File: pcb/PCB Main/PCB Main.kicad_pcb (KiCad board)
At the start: 4 copper layers, 64.1 x 56.5 mm, 81 parts, among them CN1 Conn_01x07, CN2 Conn_01x02, CN3 Conn_01x02, CN4 Conn_01x04, CN5 Conn_01x04, CN6 Conn_01x03, CN7 Conn_01x03, CN8 Conn_01x03, CN9 Conn_01x02, J1 Conn_01x03, Q1 AO3401A, SW1 SW_Reset, U1 STM32WB55RGVx, U2 AEM10941, U3 INA3221, U4 MB85RS256B, X1 32MHz, X2 32.768kHz

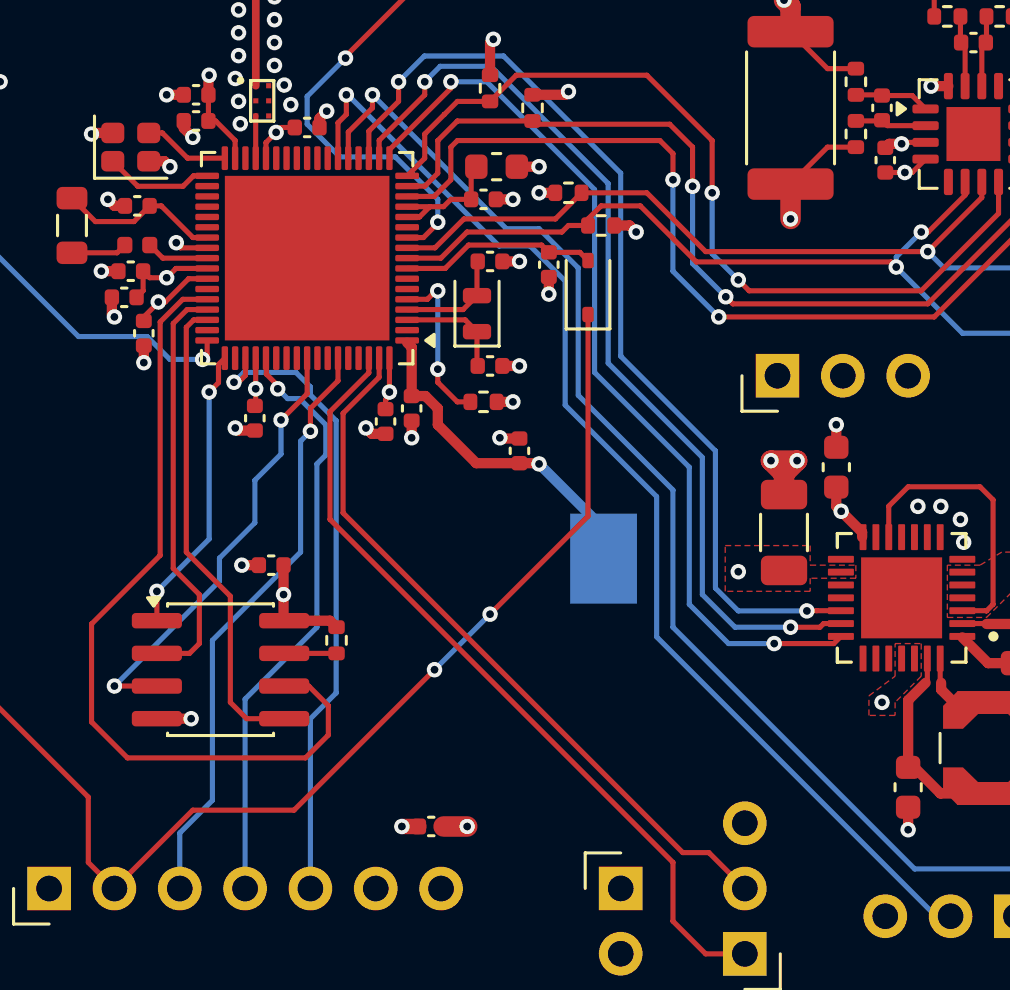
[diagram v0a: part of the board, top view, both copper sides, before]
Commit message: retoques
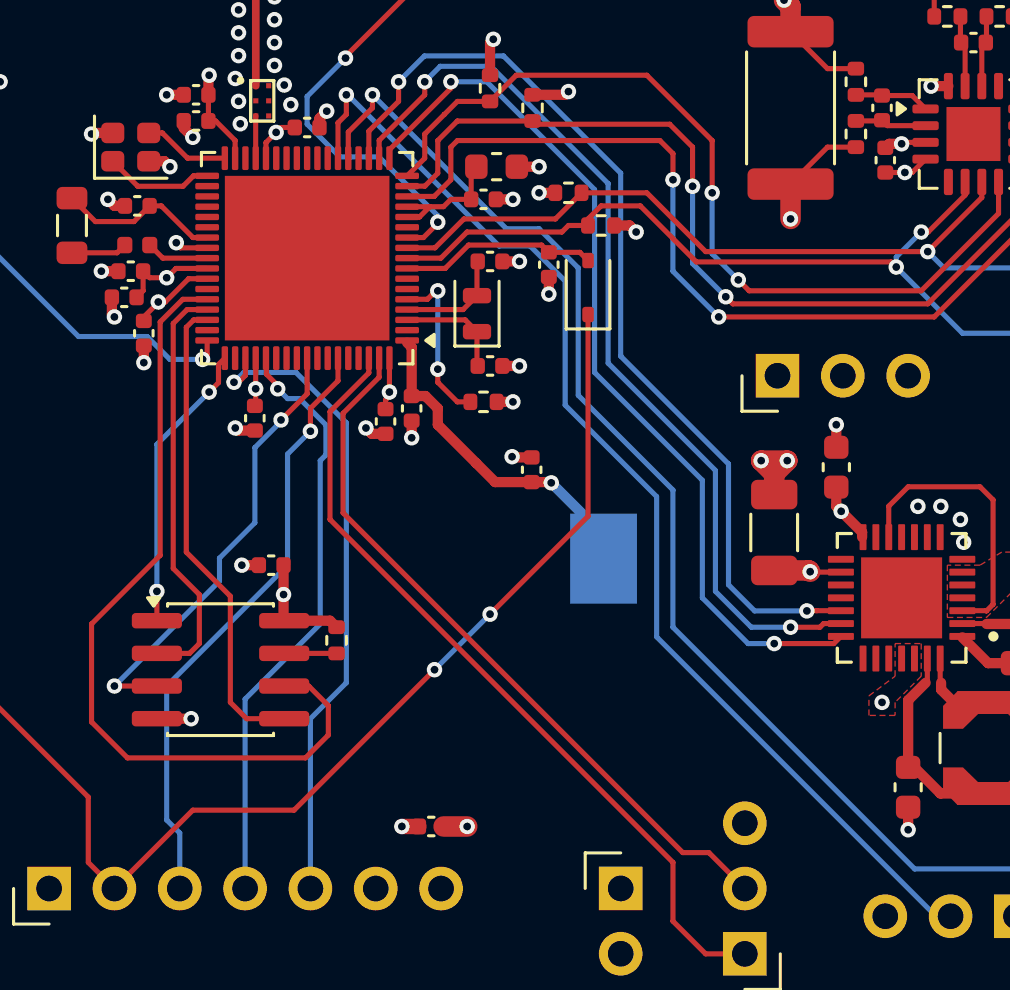
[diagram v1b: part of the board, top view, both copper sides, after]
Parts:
- moved C26 0.88 mm to (50.4, 49.1)
- moved C9 0.38 mm to (59.8, 51.6)
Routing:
- net /Power Management/BATT: track 4.62 -> 7.24 mm
- removed copper zone on F.Cu, net /Power Management/BATT
